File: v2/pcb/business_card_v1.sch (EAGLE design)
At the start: 31 parts, among them SW1 SPST_TACT-KMR2

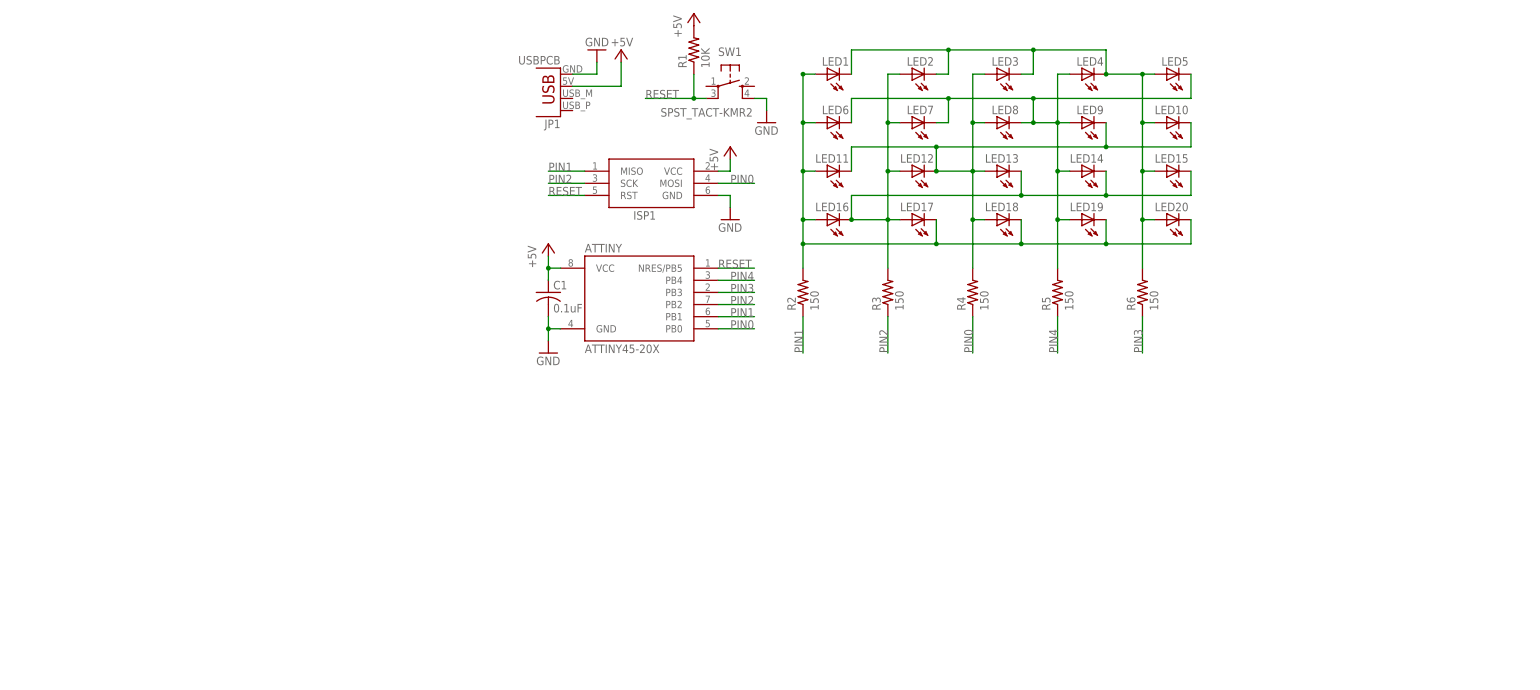
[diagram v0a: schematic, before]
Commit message: get the led layout right
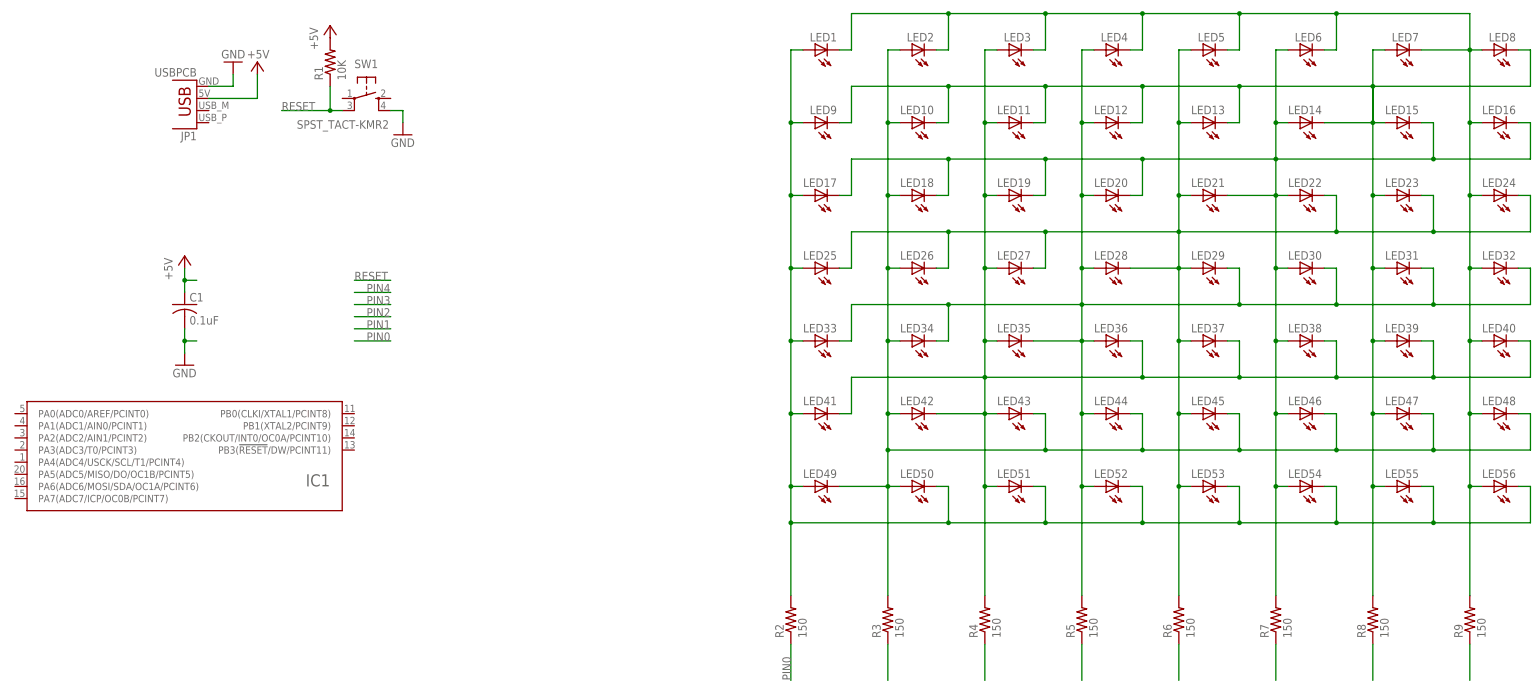
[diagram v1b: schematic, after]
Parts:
- removed ATTINY: ATTINY45-20X, _hhn_attiny25_45_85:ATTINY45-20X
- removed ISP1: AVRISP-6, adafruit:AVRISP-6
- added IC1: (no value), atmel_tiny24-44-84tiny48-88mega48-88-168-328:ATTINY24/44/84-MU
- added LED21, LED22, LED23, LED24, LED25, LED26, LED27, LED28, LED29, LED30, LED31, LED32, LED33, LED34, LED35, LED36, LED37, LED38, LED39, LED40, LED41, LED42, LED43, LED44, LED45, LED46, LED47, LED48, LED49, LED50, LED51, LED52, LED53, LED54, LED55, LED56: (no value), led:LEDCHIPLED_0805
- added R7, R8, R9: 150, resistor:R-US_R0603
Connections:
- removed net PIN1: ATTINY.PB1, ISP1.MISO, R2.1
- removed net PIN2: ATTINY.PB2, ISP1.SCK, R3.1
- removed net PIN3: ATTINY.PB3, R6.1
- removed net PIN4: ATTINY.PB4, R5.1
- new net N$10: R4.1
- new net N$11: R5.1
- new net N$15: LED10.C, LED11.C, LED12.C, LED13.C, LED14.C, LED15.A, LED23.A, LED31.A, LED39.A, LED47.A, LED55.A, LED7.A, LED8.C, LED9.C, R8.2
- new net N$2: LED10.A, LED18.A, LED2.A, LED26.A, LED34.A, LED42.A, LED43.C, LED44.C, LED45.C, LED46.C, LED47.C, LED48.C, LED49.C, LED50.A, R3.2
- new net N$3: LED11.A, LED19.A, LED27.A, LED3.A, LED35.A, LED36.C, LED37.C, LED38.C, LED39.C, LED40.C, LED41.C, LED42.C, LED43.A, LED51.A, R4.2
- new net N$31: LED14.A, LED15.C, LED16.C, LED17.C, LED18.C, LED19.C, LED20.C, LED21.C, LED22.A, LED30.A, LED38.A, LED46.A, LED54.A, LED6.A, R7.2
- new net N$34: LED13.A, LED21.A, LED22.C, LED23.C, LED24.C, LED25.C, LED26.C, LED27.C, LED28.C, LED29.A, LED37.A, LED45.A, LED5.A, LED53.A, R6.2
- new net N$4: LED12.A, LED20.A, LED28.A, LED29.C, LED30.C, LED31.C, LED32.C, LED33.C, LED34.C, LED35.C, LED36.A, LED4.A, LED44.A, LED52.A, R5.2
- new net N$5: R8.1
- new net N$8: LED1.C, LED16.A, LED2.C, LED24.A, LED3.C, LED32.A, LED4.C, LED40.A, LED48.A, LED5.C, LED56.A, LED6.C, LED7.C, LED8.A, R9.2
- net +5V: no longer ATTINY.VCC, ISP1.VCC
- net GND: no longer ATTINY.GND, ISP1.GND
- net N$1: now also LED17.A, LED25.A, LED33.A, LED41.A, LED49.A, LED50.C, LED51.C, LED52.C, LED53.C, LED54.C, LED55.C, LED56.C, LED9.A; no longer LED11.A, LED16.A, LED17.C, LED18.C, LED19.C, LED20.C, LED6.A
- net N$12: now also R6.1; no longer LED10.C, LED11.C, LED12.C, LED13.A, LED18.A, LED3.A, LED8.A, LED9.C, R4.2
- net N$13: now also R7.1; no longer LED12.A, LED13.C, LED14.C, LED15.C, LED16.C, LED17.A, LED2.A, LED7.A, R3.2
- net N$6: now also R9.1; no longer LED1.C, LED10.A, LED15.A, LED2.C, LED20.A, LED3.C, LED4.C, LED5.A, R6.2
- net N$9: now also R3.1; no longer LED14.A, LED19.A, LED4.A, LED5.C, LED6.C, LED7.C, LED8.C, LED9.A, R5.2
- net PIN0: now also R2.1; no longer ATTINY.PB0, ISP1.MOSI, R4.1
- net RESET: no longer ATTINY.NRES/PB5, ISP1.RST
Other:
- moved on the sheet: C1, JP1, LED1, LED10, LED11, LED12, LED13, LED14, LED15, LED16, LED17, LED18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
